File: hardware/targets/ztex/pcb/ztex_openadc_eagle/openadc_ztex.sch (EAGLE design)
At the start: 197 parts, among them CON3 JTAG, CON6 USB-FPGA1.15, IC1 AOZ1021, IC2 AOZ1021, IC3 AOZ1094, IC4 AOZ1021, IC5 AT90USB162A, T1 TC1-1T, U1 AD9215BRUZ, U2 AD8331, U3 LP3985IM5-3.0, U5 CDCE906PW, U6 TXB0104PWR, U7 TXB0108PWR, U8 SN74LVC1T45DBVT, U9 SN74LVC1T45DBVT, X1 SMA-142-0711-821/826, X2 SMA-142-0711-821/826, X3 SMA-142-0711-821/826, X4 SMA-142-0711-821/826, X5 PN61729-S

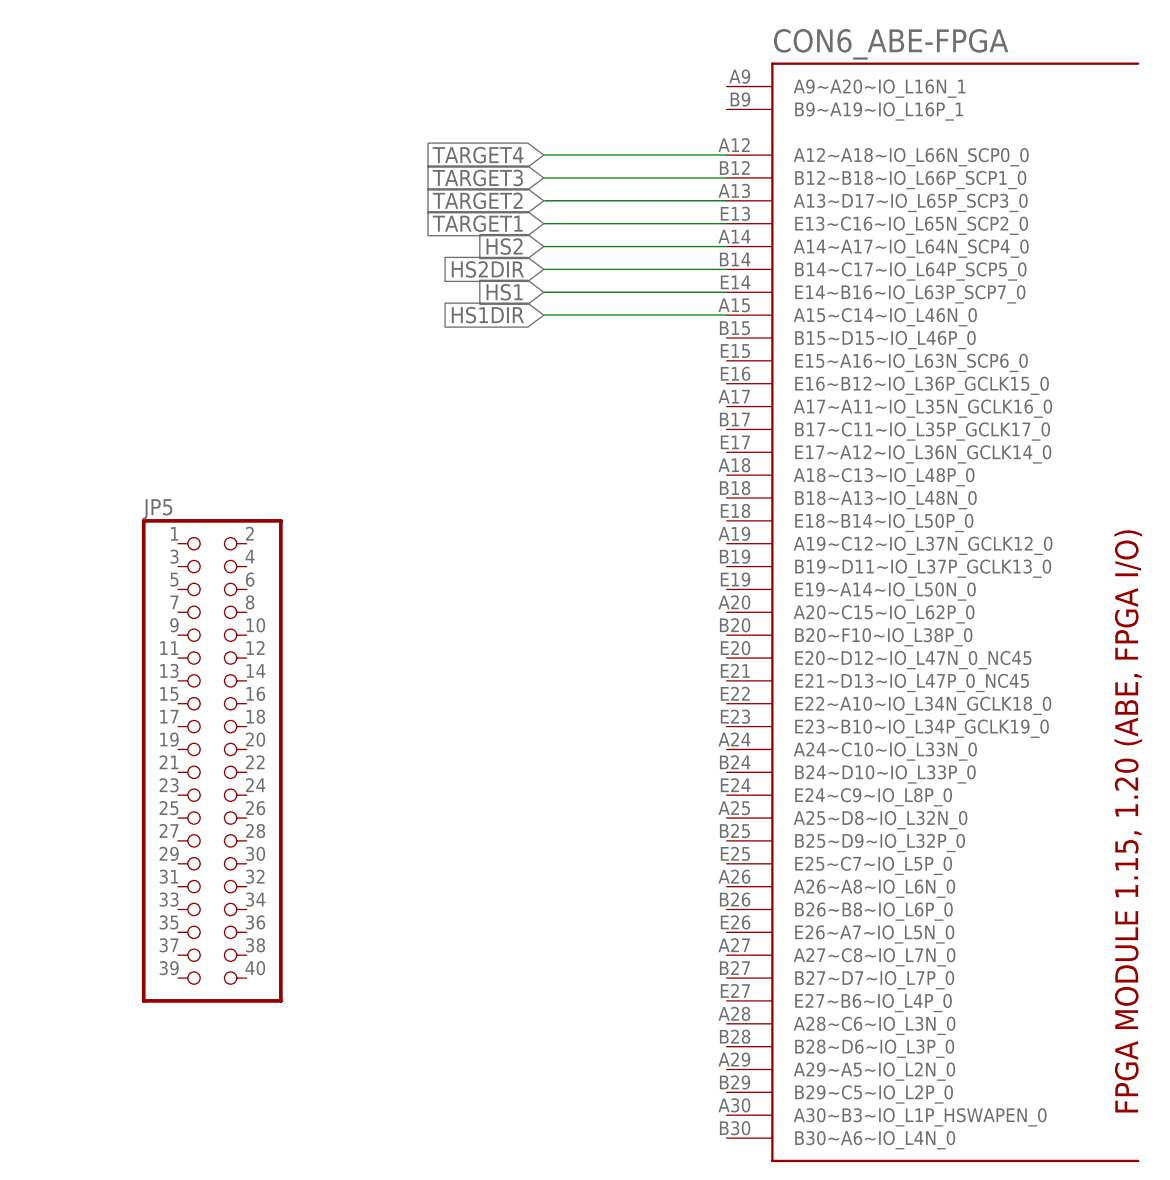
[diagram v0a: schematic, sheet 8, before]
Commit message: Finished ZTEX Board
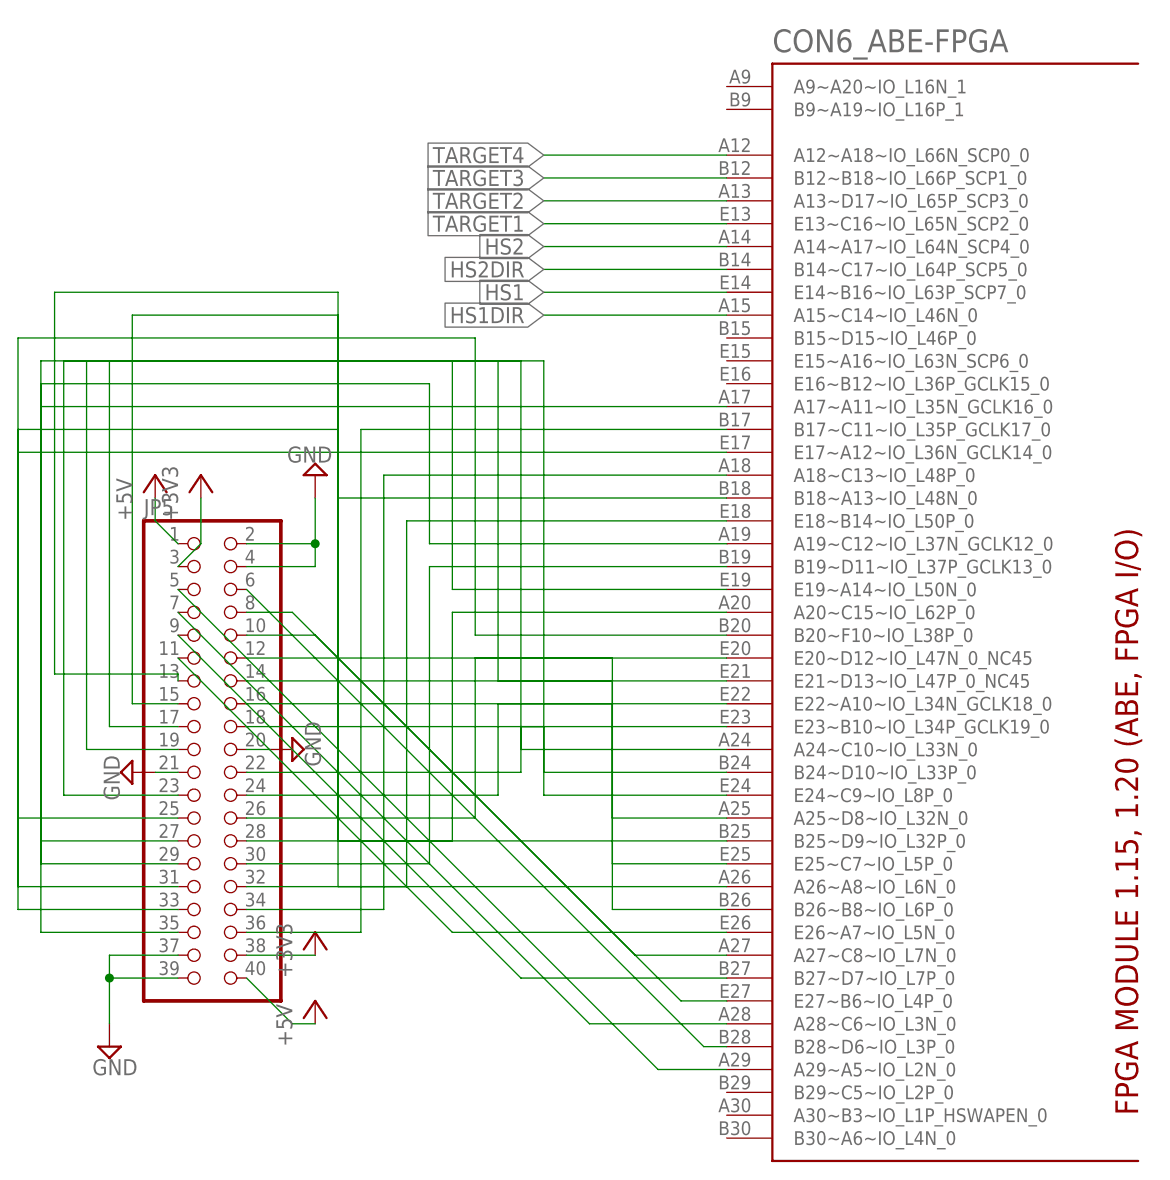
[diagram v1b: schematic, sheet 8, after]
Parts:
- added C81, C82, C83: (no value), rcl:C-EUC0603
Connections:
- removed net AGND: C45.2, C62.2, D3.A
- removed net DGND: X3.2
- removed net VCCIO: U6.VCCA, U8.VCCA, U9.VCCA
- new net N$119: CON6_ABE-FPGA.B17~C11~IO_L35P_GCLK17_0, JP5.36
- new net N$120: CON6_ABE-FPGA.E17~A12~IO_L36N_GCLK14_0, JP5.33
- new net N$121: CON6_ABE-FPGA.A18~C13~IO_L48P_0, JP5.34
- new net N$124: CON6_ABE-FPGA.B18~A13~IO_L48N_0, JP5.31
- new net N$125: CON6_ABE-FPGA.E18~B14~IO_L50P_0, JP5.32
- new net N$126: CON6_ABE-FPGA.A19~C12~IO_L37N_GCLK12_0, JP5.29
- new net N$127: CON6_ABE-FPGA.B19~D11~IO_L37P_GCLK13_0, JP5.30
- new net N$128: CON6_ABE-FPGA.E19~A14~IO_L50N_0, JP5.27
- new net N$129: CON6_ABE-FPGA.A20~C15~IO_L62P_0, JP5.28
- new net N$130: CON6_ABE-FPGA.B20~F10~IO_L38P_0, JP5.25
- new net N$131: CON6_ABE-FPGA.E20~D12~IO_L47N_0_NC45, JP5.26
- new net N$132: CON6_ABE-FPGA.E21~D13~IO_L47P_0_NC45, JP5.23
- new net N$133: CON6_ABE-FPGA.E22~A10~IO_L34N_GCLK18_0, JP5.24
- new net N$134: CON6_ABE-FPGA.E23~B10~IO_L34P_GCLK19_0, JP5.22
- new net N$135: CON6_ABE-FPGA.A24~C10~IO_L33N_0, JP5.19
- new net N$136: CON6_ABE-FPGA.B24~D10~IO_L33P_0, JP5.18
- new net N$137: CON6_ABE-FPGA.E24~C9~IO_L8P_0, JP5.17
- new net N$138: CON6_ABE-FPGA.A25~D8~IO_L32N_0, JP5.16
- new net N$139: CON6_ABE-FPGA.B25~D9~IO_L32P_0, JP5.15
- new net N$140: CON6_ABE-FPGA.E25~C7~IO_L5P_0, JP5.14
- new net N$141: CON6_ABE-FPGA.A26~A8~IO_L6N_0, JP5.13
- new net N$142: CON6_ABE-FPGA.B26~B8~IO_L6P_0, JP5.12
- new net N$143: CON6_ABE-FPGA.E26~A7~IO_L5N_0, JP5.11
- new net N$144: CON6_ABE-FPGA.A27~C8~IO_L7N_0, JP5.10
- new net N$145: CON6_ABE-FPGA.B27~D7~IO_L7P_0, JP5.9
- new net N$146: CON6_ABE-FPGA.E27~B6~IO_L4P_0, JP5.8
- new net N$147: CON6_ABE-FPGA.A28~C6~IO_L3N_0, JP5.7
- new net N$148: CON6_ABE-FPGA.B28~D6~IO_L3P_0, JP5.6
- new net N$149: CON6_ABE-FPGA.A29~A5~IO_L2N_0, JP5.5
- new net N$66: CON6_ABE-FPGA.A17~A11~IO_L35N_GCLK16_0, JP5.35
- net +3V3: now also C81.1, C82.1, C83.1, JP5.3, JP5.38, U6.VCCA, U8.VCCA, U9.VCCA
- net +5V: now also JP5.1, JP5.40
- net GND: now also C45.2, C62.2, C81.2, C82.2, C83.2, D3.A, JP5.2, JP5.20, JP5.21, JP5.37, JP5.39, JP5.4, X3.2

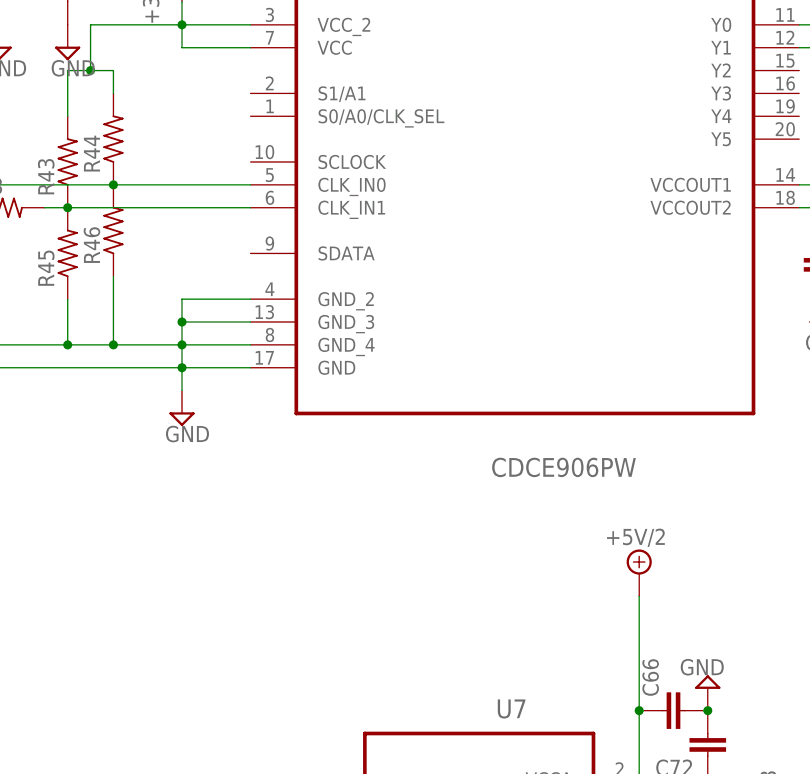
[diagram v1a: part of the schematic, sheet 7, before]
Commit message: Round-2 ZTEX board, fix a few more errors
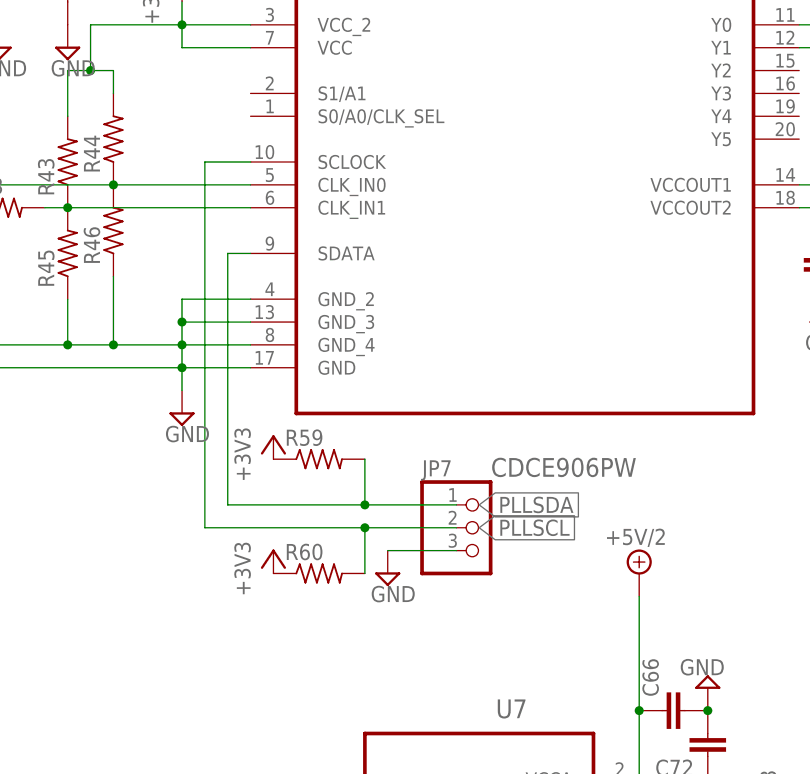
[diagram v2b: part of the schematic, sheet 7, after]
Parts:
- added JP7: (no value), pinhead:PINHD-1X3
- added R59, R60: (no value), resistor:R-US_R0603
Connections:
- removed net N$149: CON6_ABE-FPGA.A29~A5~IO_L2N_0, JP5.5
- new net PLLSCL: CON6_ABE-FPGA.A29~A5~IO_L2N_0, JP7.2, R60.2, U5.SCLOCK
- new net PLLSDA: CON6_ABE-FPGA.B29~C5~IO_L2P_0, JP7.1, R59.2, U5.SDATA
- net +3V3: now also R59.1, R60.1
- net GND: now also JP7.3
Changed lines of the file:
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@@
 <part name="+3V33" library="supply1" deviceset="+3V3" device=""/>
 <part name="SUPPLY38" library="supply2" deviceset="GND" device=""/>
+<part name="R59" library="resistor" deviceset="R-US_" device="R0603"/>
+<part name="R60" library="resistor" deviceset="R-US_" device="R0603"/>
+<part name="+3V34" library="supply1" deviceset="+3V3" device=""/>
+<part name="+3V35" library="supply1" deviceset="+3V3" device=""/>
+<part name="JP7" library="pinhead" deviceset="PINHD-1X3" device=""/>
+<part name="SUPPLY113" library="supply2" deviceset="GND" device=""/>
 </parts>
 <sheets>
@@
 <instance part="+3V31" gate="G$1" x="193.04" y="180.34"/>
 <instance part="SUPPLY38" gate="GND" x="15.24" y="162.56"/>
+<instance part="R59" gate="G$1" x="81.28" y="124.46"/>
+<instance part="R60" gate="G$1" x="81.28" y="111.76"/>
+<instance part="+3V34" gate="G$1" x="76.2" y="127"/>
+<instance part="+3V35" gate="G$1" x="76.2" y="114.3"/>
+<instance part="JP7" gate="A" x="99.06" y="116.84"/>
+<instance part="SUPPLY113" gate="GND" x="88.9" y="111.76"/>
 </instances>
 <busses>
@@
 <pinref part="SUPPLY38" gate="GND" pin="GND"/>
 </segment>
+<segment>
+<pinref part="JP7" gate="A" pin="3"/>
+<pinref part="SUPPLY113" gate="GND" pin="GND"/>
+<wire x1="88.9" y1="114.3" x2="96.52" y2="114.3" width="0.1524" layer="91"/>
+</segment>
 </net>
 <net name="N$93" class="0">
@@
 <pinref part="+3V31" gate="G$1" pin="+3V3"/>
 </segment>
+<segment>
+<pinref part="R59" gate="G$1" pin="1"/>
+<pinref part="+3V34" gate="G$1" pin="+3V3"/>
+</segment>
+<segment>
+<pinref part="R60" gate="G$1" pin="1"/>
+<pinref part="+3V35" gate="G$1" pin="+3V3"/>
+</segment>
 </net>
 <net name="N$89" class="0">
@@
 </segment>
 </net>
+<net name="PLLSDA" class="0">
+<segment>
+<pinref part="U5" gate="A" pin="SDATA"/>
+<wire x1="73.66" y1="147.32" x2="71.12" y2="147.32" width="0.1524" layer="91"/>
+<wire x1="71.12" y1="147.32" x2="71.12" y2="119.38" width="0.1524" layer="91"/>
+<wire x1="71.12" y1="119.38" x2="86.36" y2="119.38" width="0.1524" layer="91"/>
+<pinref part="R59" gate="G$1" pin="2"/>
+<wire x1="86.36" y1="119.38" x2="86.36" y2="124.46" width="0.1524" layer="91"/>
+<pinref part="JP7" gate="A" pin="1"/>
+<wire x1="96.52" y1="119.38" x2="86.36" y2="119.38" width="0.1524" layer="91"/>
+<junction x="86.36" y="119.38"/>
+<label x="99.06" y="119.38" size="1.778" layer="95" xref="yes"/>
+</segment>
+</net>
+<net name="PLLSCL" class="0">
+<segment>
+<pinref part="U5" gate="A" pin="SCLOCK"/>
+<wire x1="73.66" y1="157.48" x2="68.58" y2="157.48" width="0.1524" layer="91"/>
+<wire x1="68.58" y1="157.48" x2="68.58" y2="116.84" width="0.1524" layer="91"/>
+<wire x1="68.58" y1="116.84" x2="86.36" y2="116.84" width="0.1524" layer="91"/>
+<pinref part="R60" gate="G$1" pin="2"/>
+<wire x1="86.36" y1="111.76" x2="86.36" y2="116.84" width="0.1524" layer="91"/>
+<pinref part="JP7" gate="A" pin="2"/>
+<wire x1="86.36" y1="116.84" x2="96.52" y2="116.84" width="0.1524" layer="91"/>
+<junction x="86.36" y="116.84"/>
+<label x="99.06" y="116.84" size="1.778" layer="95" xref="yes"/>
+</segment>
+</net>
 </nets>
 </sheet>
@@
 </segment>
 </net>
-<net name="N$149" class="0">
-<segment>
-<pinref part="CON6" gate="_ABE-FPGA" pin="A29~A5~IO_L2N_0"/>
-<pinref part="JP5" gate="A" pin="5"/>
-<wire x1="165.1" y1="63.5" x2="157.48" y2="63.5" width="0.1524" layer="91"/>
-<wire x1="157.48" y1="63.5" x2="104.14" y2="116.84" width="0.1524" layer="91"/>
-</segment>
-</net>
 <net name="+5V" class="0">
 <segment>
@@
 </segment>
 </net>
+<net name="PLLSDA" class="0">
+<segment>
+<pinref part="CON6" gate="_ABE-FPGA" pin="B29~C5~IO_L2P_0"/>
+<wire x1="165.1" y1="60.96" x2="152.4" y2="60.96" width="0.1524" layer="91"/>
+<label x="152.4" y="60.96" size="1.778" layer="95" rot="R180" xref="yes"/>
+</segment>
+</net>
+<net name="PLLSCL" class="0">
+<segment>
+<pinref part="CON6" gate="_ABE-FPGA" pin="A29~A5~IO_L2N_0"/>
+<wire x1="165.1" y1="63.5" x2="152.4" y2="63.5" width="0.1524" layer="91"/>
+<label x="152.4" y="63.5" size="1.778" layer="95" rot="R180" xref="yes"/>
+</segment>
+</net>
